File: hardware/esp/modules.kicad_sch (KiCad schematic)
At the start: 41 parts, among them J5 Conn_Coaxial, J6 Conn_01x09_Pin, J7 Conn_01x06_Pin, J8 Conn_01x09_Pin, U4 VL53L0X, U5 NRF24L01, U6 BME280, Y1 16MHz

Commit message: Updating schematic, BOM, and component placement on PCB
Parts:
- C17: footprint Capacitor_SMD:C_0603_1608Metric -> Capacitor_SMD:C_0805_2012Metric
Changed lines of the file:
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@@
 			)
 		)
-		(property "Footprint" "Capacitor_SMD:C_0603_1608Metric"
+		(property "Footprint" "Capacitor_SMD:C_0805_2012Metric"
 			(at 122.2248 25.4 0)
 			(hide yes)

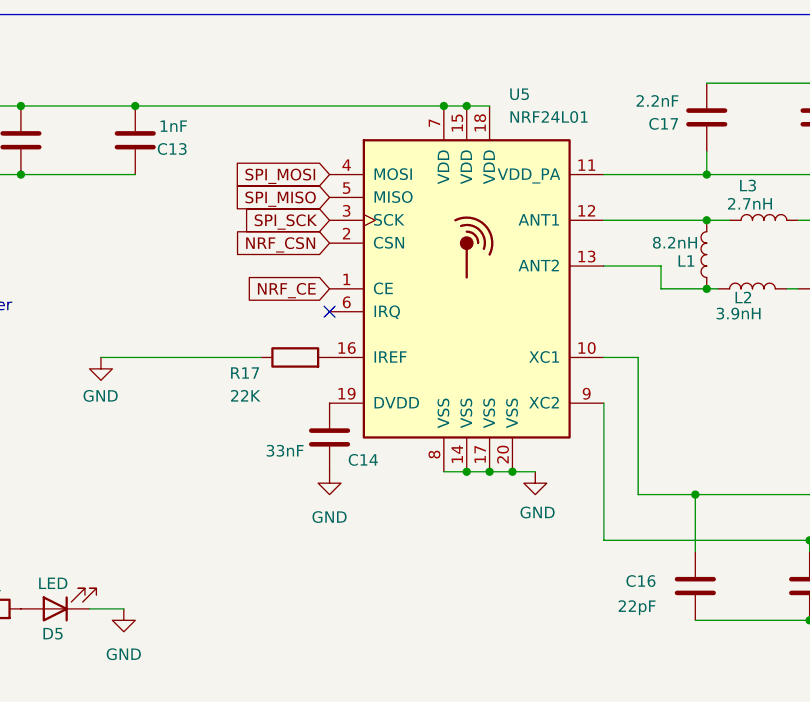
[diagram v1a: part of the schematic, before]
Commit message: Updating PCB
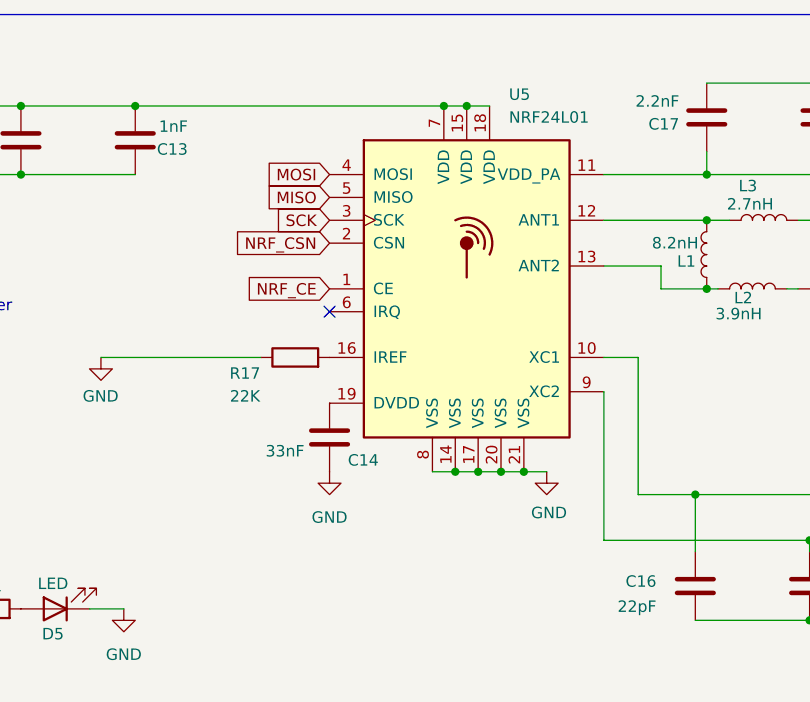
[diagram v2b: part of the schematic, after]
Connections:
- net GND: now also U5.21 (VSS)
- net SPI_MISO renamed MISO
- net SPI_MOSI renamed MOSI
- net SPI_SCK renamed SCK
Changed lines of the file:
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@@
 	)
 	(junction
-		(at 96.52 68.58)
-		(diameter 0)
-		(color 0 0 0 0)
-	)
-	(junction
 		(at 228.6 50.8)
 		(diameter 0)
@@
 	)
 	(junction
-		(at 101.6 68.58)
-		(diameter 0)
-		(color 0 0 0 0)
-	)
-	(junction
 		(at 134.62 76.2)
 		(diameter 0)
@@
 	)
 	(junction
+		(at 95.25 68.58)
+		(diameter 0)
+		(color 0 0 0 0)
+	)
+	(junction
+		(at 100.33 68.58)
+		(diameter 0)
+		(color 0 0 0 0)
+	)
+	(junction
 		(at 156.21 85.09)
 		(diameter 0)
@@
 	)
 	(junction
-		(at 99.06 68.58)
-		(diameter 0)
-		(color 0 0 0 0)
-	)
-	(junction
 		(at 96.52 27.94)
 		(diameter 0)
@@
 	)
 	(junction
+		(at 102.87 68.58)
+		(diameter 0)
+		(color 0 0 0 0)
+	)
+	(junction
 		(at 134.62 85.09)
 		(diameter 0)
@@
 		(color 0 0 0 0)
 	)
+	(junction
+		(at 97.79 68.58)
+		(diameter 0)
+		(color 0 0 0 0)
+	)
 	(no_connect
 		(at 226.06 62.23)
@@
 	(wire
 		(pts
+			(xy 97.79 68.58) (xy 95.25 68.58)
+		)
+		(stroke
+			(width 0)
+			(type default)
+		)
+	)
+	(wire
+		(pts
 			(xy 46.99 35.56) (xy 59.69 35.56)
 		)
@@
 	(wire
 		(pts
+			(xy 111.76 59.69) (xy 111.76 76.2)
+		)
+		(stroke
+			(width 0)
+			(type default)
+		)
+	)
+	(wire
+		(pts
 			(xy 234.95 133.35) (xy 234.95 140.97)
 		)
@@
 	(wire
 		(pts
+			(xy 95.25 68.58) (xy 92.71 68.58)
+		)
+		(stroke
+			(width 0)
+			(type default)
+		)
+	)
+	(wire
+		(pts
 			(xy 116.84 156.21) (xy 113.03 156.21)
 		)
@@
 	(wire
 		(pts
-			(xy 111.76 60.96) (xy 111.76 76.2)
+			(xy 100.33 68.58) (xy 97.79 68.58)
 		)
 		(stroke
@@
 	(wire
 		(pts
+			(xy 102.87 68.58) (xy 100.33 68.58)
+		)
+		(stroke
+			(width 0)
+			(type default)
+		)
+	)
+	(wire
+		(pts
 			(xy 73.66 165.1) (xy 80.01 165.1)
 		)
@@
 	(wire
 		(pts
+			(xy 102.87 68.58) (xy 105.41 68.58)
+		)
+		(stroke
+			(width 0)
+			(type default)
+		)
+	)
+	(wire
+		(pts
 			(xy 121.92 85.09) (xy 134.62 85.09)
 		)
@@
 	(wire
 		(pts
-			(xy 93.98 68.58) (xy 101.6 68.58)
-		)
-		(stroke
-			(width 0)
-			(type default)
-		)
-	)
-	(wire
-		(pts
 			(xy 96.52 27.94) (xy 99.06 27.94)
 		)
@@
 	(wire
 		(pts
-			(xy 101.6 68.58) (xy 104.14 68.58)
-		)
-		(stroke
-			(width 0)
-			(type default)
-		)
-	)
-	(wire
-		(pts
 			(xy 215.9 72.39) (xy 226.06 72.39)
 		)
@@
 		)
 	)
-	(global_label "SPI_MOSI"
+	(global_label "MOSI"
 		(shape input)
 		(at 81.28 35.56 180)
@@
 		)
 		(property "Intersheetrefs" "${INTERSHEET_REFS}"
-			(at 69.0419 35.56 0)
+			(at 73.6986 35.56 0)
 			(hide yes)
 			(show_name no)
@@
 		)
 	)
-	(global_label "SPI_MISO"
+	(global_label "MISO"
 		(shape input)
 		(at 81.28 38.1 180)
@@
 		)
 		(property "Intersheetrefs" "${INTERSHEET_REFS}"
-			(at 69.6467 38.1 0)
+			(at 73.6986 38.1 0)
 			(hide yes)
 			(show_name no)
@@
 		)
 	)
-	(global_label "SPI_SCK"
+	(global_label "SCK"
 		(shape input)
 		(at 81.28 40.64 180)
@@
 		)
 		(property "Intersheetrefs" "${INTERSHEET_REFS}"
-			(at 69.0419 40.64 0)
+			(at 74.5453 40.64 0)
 			(hide yes)
 			(show_name no)
@@
 		(pin "20"
 		)
+		(pin "21"
+		)
 		(instances
 			(project "esp"
@@
 	(symbol
 		(lib_id "power:GND")
-		(at 104.14 68.58 0)
+		(at 105.41 68.58 0)
 		(unit 1)
 		(body_style 1)
@@
 		(dnp no)
 		(property "Reference" "#PWR030"
-			(at 104.14 74.93 0)
+			(at 105.41 74.93 0)
 			(hide yes)
 			(show_name no)
@@
 		)
 		(property "Value" "GND"
-			(at 104.394 73.152 0)
+			(at 105.664 73.152 0)
 			(show_name no)
 			(do_not_autoplace no)
@@
 		)
 		(property "Footprint" ""
-			(at 104.14 68.58 0)
+			(at 105.41 68.58 0)
 			(hide yes)
 			(show_name no)
@@
 		)
 		(property "Datasheet" ""
-			(at 104.14 68.58 0)
+			(at 105.41 68.58 0)
 			(hide yes)
 			(show_name no)
@@
 		)
 		(property "Description" "Power symbol creates a global label with name \"GND\" , ground"
-			(at 104.14 68.58 0)
+			(at 105.41 68.58 0)
 			(hide yes)
 			(show_name no)
